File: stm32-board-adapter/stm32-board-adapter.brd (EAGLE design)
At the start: 41.3 x 51.3 mm, 35 parts, among them J2 22-05-7048-04, J3 22-05-7048-04, J4 22-05-7048-04, J5 22-05-7048-04

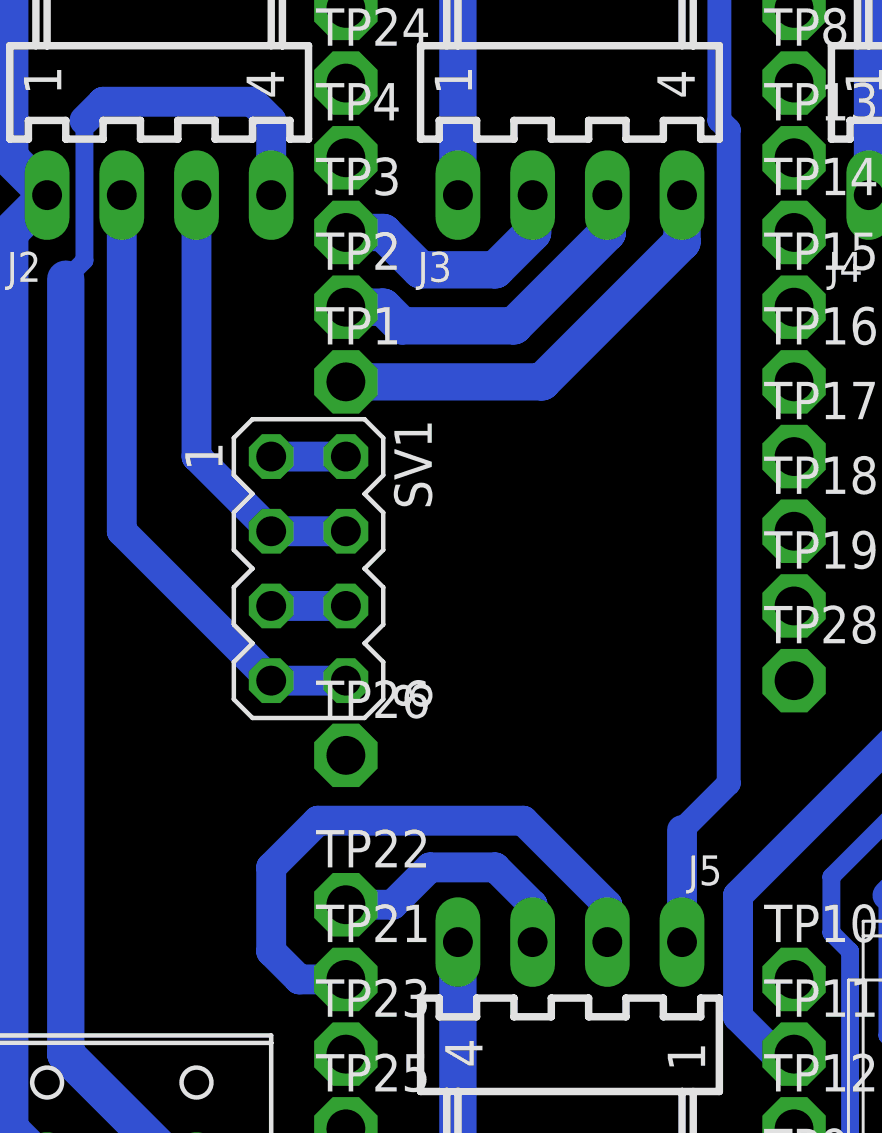
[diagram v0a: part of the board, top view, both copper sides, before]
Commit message: stm32-board-adapter enhancements
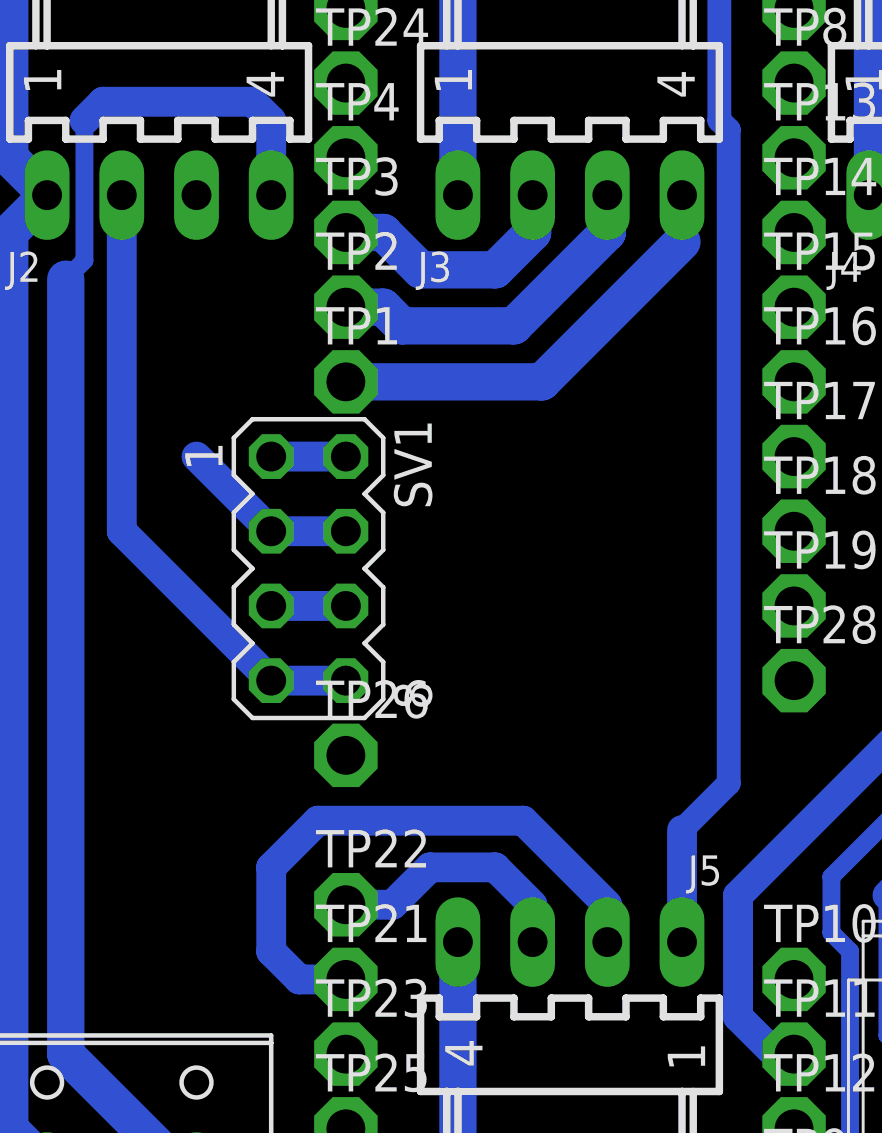
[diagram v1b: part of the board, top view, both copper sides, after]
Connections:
- net A1 renamed PA1_RTS2
- net A2 renamed PA2_TX2
- net B10 renamed B10_SCL2_TX3
- net B11 renamed B11_SDA2_RX3
- net MOSI2 renamed B15_MOSI2
- net SCK2 renamed B13_SCK2
- new net PA3_RX2: J3.4
- new net PA5_SCK1: J2.3
- net A3: no longer J3.4
- net SCK: no longer J2.3
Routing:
- net SCK: track 15.0 -> 6.13 mm
- net A3: track 15.0 -> 13.4 mm
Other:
- board text added: "CLK_DATA"
- board text added: "CLK_DATA_2"
- board text added: "I2C / UART"
- board text added: "P_SUPP"
- board text added: "UART"
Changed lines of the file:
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@@
 <?xml version="1.0" encoding="utf-8"?>
 <!DOCTYPE eagle SYSTEM "eagle.dtd">
-<eagle version="7.4.0">
+<eagle version="7.7.0">
 <drawing>
 <settings>
@@
 <wire x1="0" y1="0" x2="41.27" y2="0" width="0.4064" layer="20"/>
 <wire x1="20.0025" y1="51.2675" x2="20" y2="51.27" width="0.4064" layer="20"/>
+<text x="13.97" y="-5.08" size="1.778" layer="48">I2C / UART</text>
+<text x="0" y="53.34" size="1.778" layer="48">CLK_DATA</text>
+<text x="16.51" y="53.34" size="1.778" layer="48">UART</text>
+<text x="27.94" y="53.34" size="1.778" layer="48">CLK_DATA_2</text>
+<text x="30.48" y="-5.08" size="1.778" layer="48">P_SUPP</text>
+<text x="0" y="-5.08" size="1.778" layer="48">P_SUPP</text>
 </plain>
 <attributes>
@@
 <contactref element="SV1" pad="4"/>
 <contactref element="SV1" pad="3"/>
-<contactref element="J2" pad="3"/>
-<wire x1="7.62" y1="38.1" x2="7.62" y2="29.21" width="1.016" layer="16"/>
 <wire x1="7.62" y1="29.21" x2="10.16" y2="26.67" width="1.016" layer="16"/>
 <wire x1="12.7" y1="26.67" x2="10.16" y2="26.67" width="1.016" layer="16"/>
 </signal>
-<signal name="SCK2">
+<signal name="B13_SCK2">
 <contactref element="J4" pad="3"/>
 <contactref element="TP9" pad="TP"/>
@@
 <wire x1="35.56" y1="21.2725" x2="29.21" y2="14.9225" width="0.6096" layer="16"/>
 </signal>
-<signal name="MOSI2">
+<signal name="B15_MOSI2">
 <contactref element="J4" pad="2"/>
 <contactref element="TP11" pad="TP"/>
@@
 <signal name="A3">
 <contactref element="TP1" pad="TP"/>
-<contactref element="J3" pad="4"/>
 <wire x1="12.7" y1="31.75" x2="19.3675" y2="31.75" width="1.27" layer="16"/>
 <wire x1="19.3675" y1="31.75" x2="24.13" y2="36.5125" width="1.27" layer="16"/>
-<wire x1="24.13" y1="36.5125" x2="24.13" y2="38.1" width="1.27" layer="16"/>
-</signal>
-<signal name="A2">
+</signal>
+<signal name="PA2_TX2">
 <contactref element="TP2" pad="TP"/>
 <contactref element="J3" pad="3"/>
@@
 <wire x1="21.59" y1="36.83" x2="21.59" y2="38.1" width="1.27" layer="16"/>
 </signal>
-<signal name="A1">
+<signal name="PA1_RTS2">
 <contactref element="TP3" pad="TP"/>
 <contactref element="J3" pad="2"/>
@@
 <contactref element="TP12" pad="TP"/>
 </signal>
-<signal name="B11">
+<signal name="B11_SDA2_RX3">
 <contactref element="TP21" pad="TP"/>
-<contactref element="J5" pad="2"/>
-<wire x1="21.59" y1="12.7" x2="21.59" y2="13.97" width="1.016" layer="16"/>
 <wire x1="21.59" y1="13.97" x2="18.7325" y2="16.8275" width="1.016" layer="16"/>
 <wire x1="18.7325" y1="16.8275" x2="11.7475" y2="16.8275" width="1.016" layer="16"/>
@@
 <wire x1="10.16" y1="12.3825" x2="11.1125" y2="11.43" width="1.016" layer="16"/>
 <wire x1="11.1125" y1="11.43" x2="12.7" y2="11.43" width="1.016" layer="16"/>
-</signal>
-<signal name="B10">
+<contactref element="J5" pad="2"/>
+<wire x1="21.59" y1="13.97" x2="21.59" y2="12.7" width="0.8128" layer="16"/>
+</signal>
+<signal name="B10_SCL2_TX3">
 <contactref element="TP22" pad="TP"/>
-<contactref element="J5" pad="3"/>
-<wire x1="19.05" y1="12.7" x2="19.05" y2="13.97" width="1.016" layer="16"/>
 <wire x1="19.05" y1="13.97" x2="17.78" y2="15.24" width="1.016" layer="16"/>
 <wire x1="17.78" y1="15.24" x2="15.5575" y2="15.24" width="1.016" layer="16"/>
 <wire x1="15.5575" y1="15.24" x2="14.2875" y2="13.97" width="1.016" layer="16"/>
 <wire x1="12.7" y1="13.97" x2="14.2875" y2="13.97" width="1.016" layer="16"/>
+<contactref element="J5" pad="3"/>
+<wire x1="19.05" y1="13.97" x2="19.05" y2="12.7" width="0.8128" layer="16"/>
 </signal>
 <signal name="N$2">
@@
 <wire x1="12.7" y1="29.21" x2="10.16" y2="29.21" width="1.016" layer="16"/>
 </signal>
+<signal name="PA3_RX2">
+<contactref element="J3" pad="4"/>
+</signal>
+<signal name="PA5_SCK1">
+<contactref element="J2" pad="3"/>
+</signal>
 </signals>
